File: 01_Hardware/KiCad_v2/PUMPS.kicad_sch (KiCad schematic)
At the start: 20 parts, among them J600 JST_B2B, J601 JST_B2B, Q600 STN3NF06L, Q601 STN3NF06L

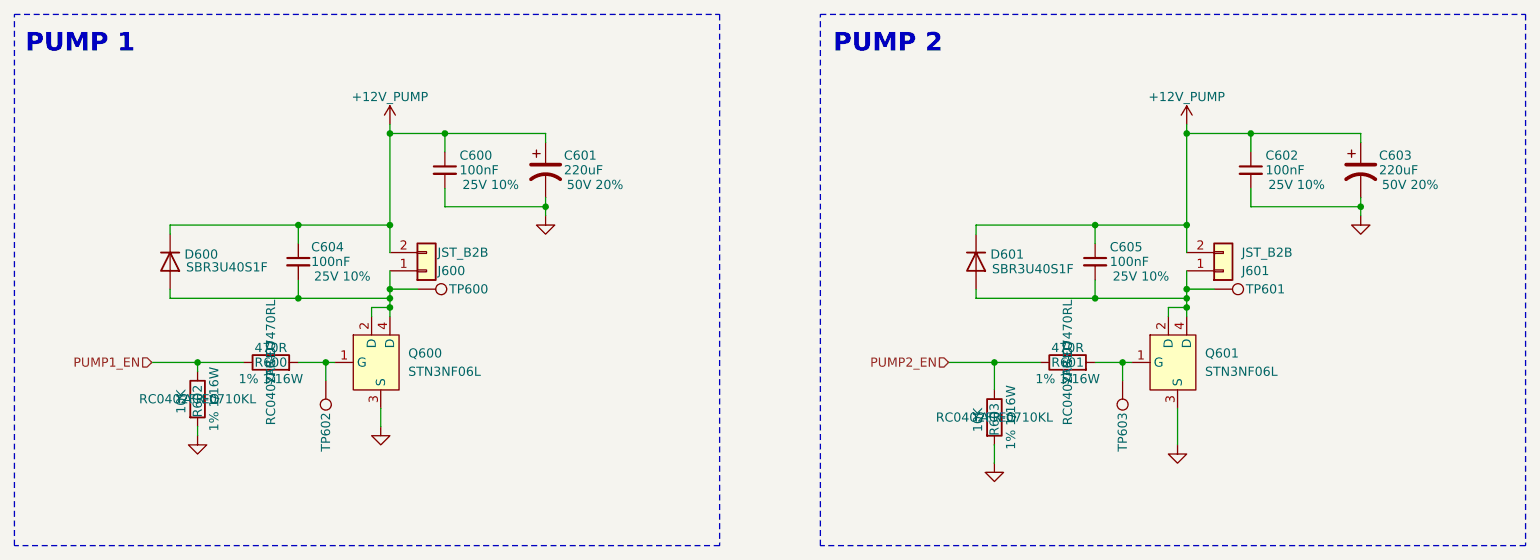
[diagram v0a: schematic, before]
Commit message: USB-C and Serial PCB routing done
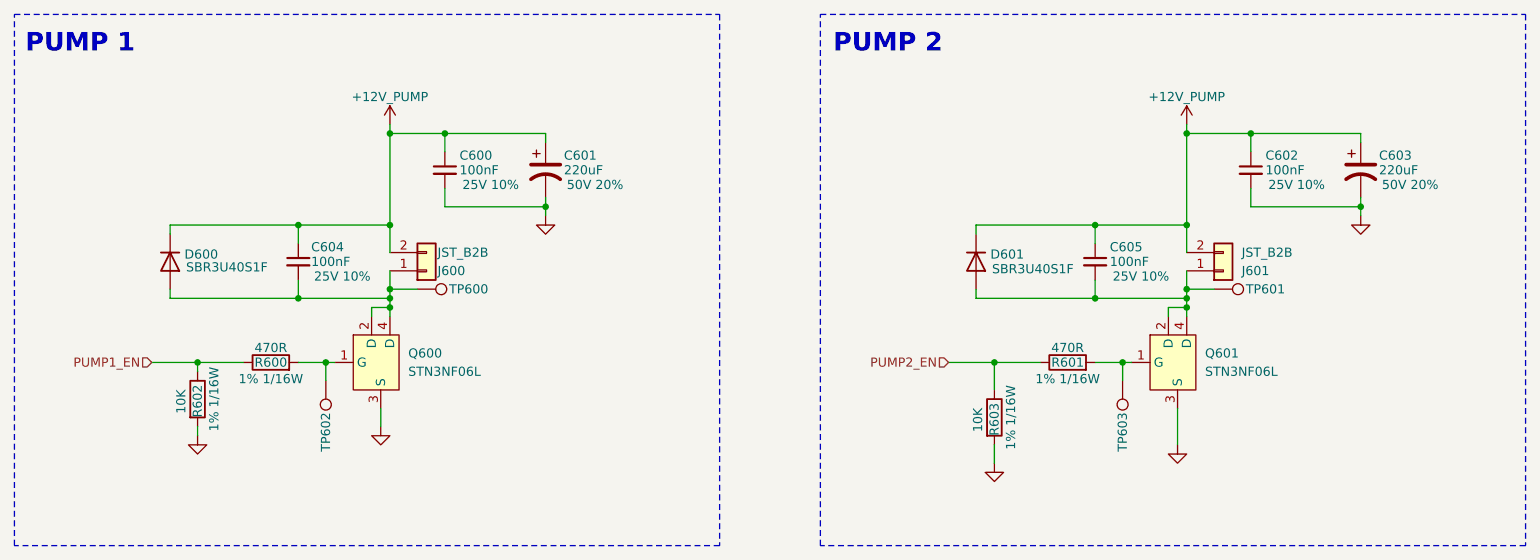
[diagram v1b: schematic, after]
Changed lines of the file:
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@@
 					(size 1.27 1.27)
 				)
+				(hide yes)
 			)
 		)
@@
 					(size 1.27 1.27)
 				)
+				(hide yes)
 			)
 		)
@@
 					(size 1.27 1.27)
 				)
+				(hide yes)
 			)
 		)
@@
 					(size 1.27 1.27)
 				)
+				(hide yes)
 			)
 		)
@@
 					(size 1.27 1.27)
 				)
+				(hide yes)
 			)
 		)
@@
 					(size 1.27 1.27)
 				)
+				(hide yes)
 			)
 		)
@@
 					(size 1.27 1.27)
 				)
+				(hide yes)
 			)
 		)
@@
 					(size 1.27 1.27)
 				)
+				(hide yes)
 			)
 		)
@@
 					(size 1.27 1.27)
 				)
+				(hide yes)
 			)
 		)
@@
 					(size 1.27 1.27)
 				)
+				(hide yes)
 			)
 		)
@@
 					(size 1.27 1.27)
 				)
+				(hide yes)
 			)
 		)
@@
 					(size 1.27 1.27)
 				)
+				(hide yes)
 			)
 		)
@@
 					(size 1.27 1.27)
 				)
+				(hide yes)
 			)
 		)
@@
 					(size 1.27 1.27)
 				)
+				(hide yes)
 			)
 		)
@@
 					(size 1.27 1.27)
 				)
+				(hide yes)
 			)
 		)
@@
 					(size 1.27 1.27)
 				)
-			)
-		)
+				(hide yes)
+			)
+		)
